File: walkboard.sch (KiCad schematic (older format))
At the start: 154 parts, among them J1 USB_C_Receptacle_USB2.0, SW1 SW_Push, U1 ATmega32U4-AU, Y1 Crystal_GND24_Small

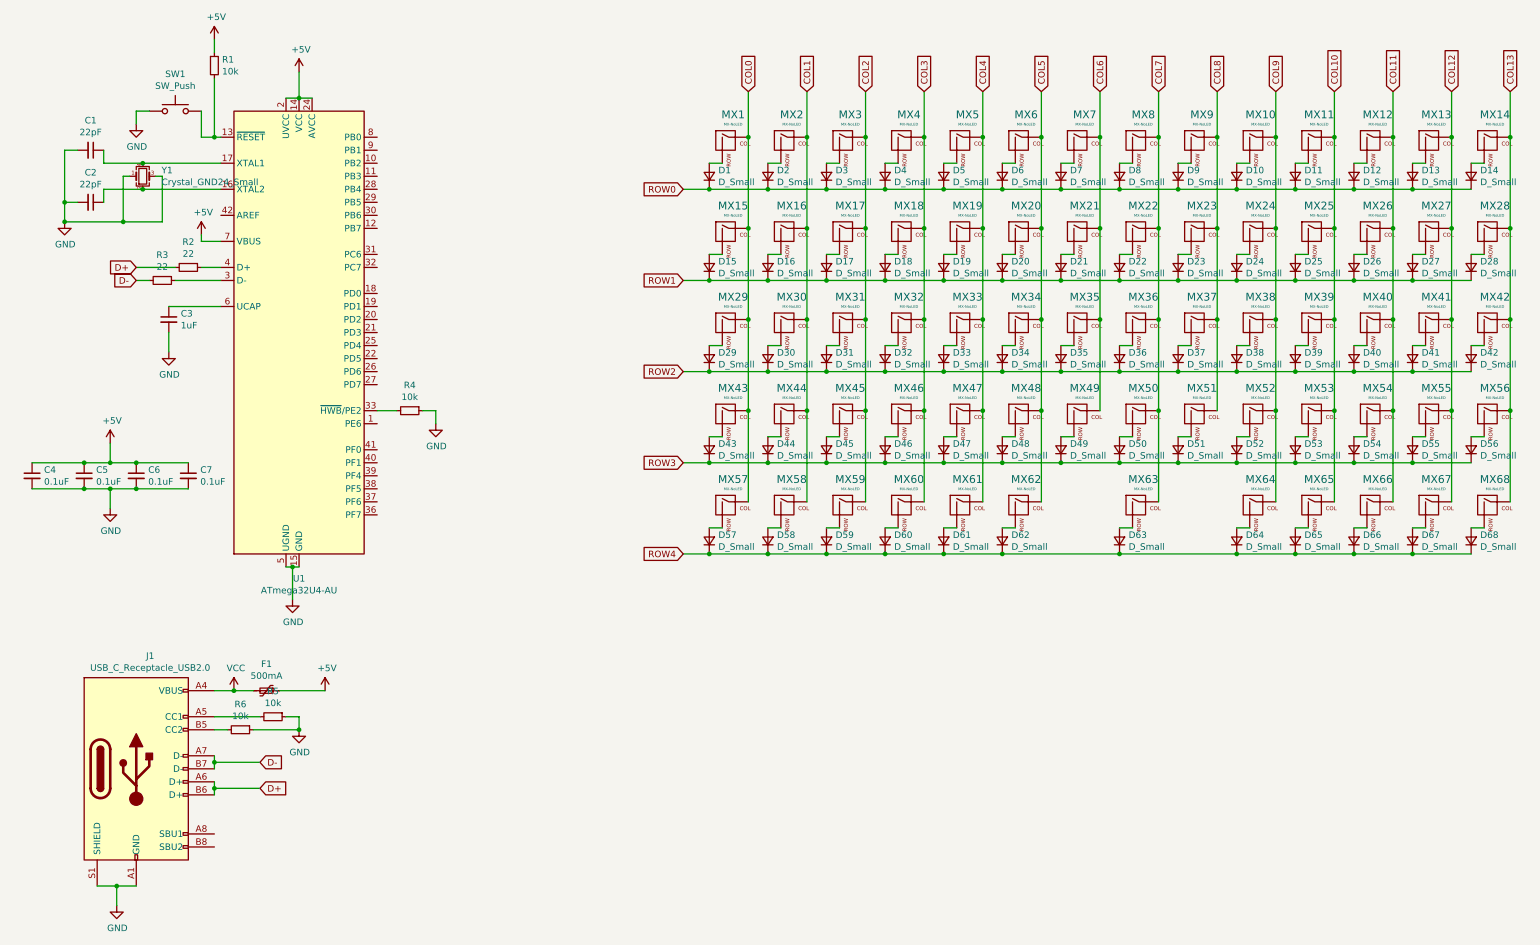
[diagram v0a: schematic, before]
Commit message: fixed
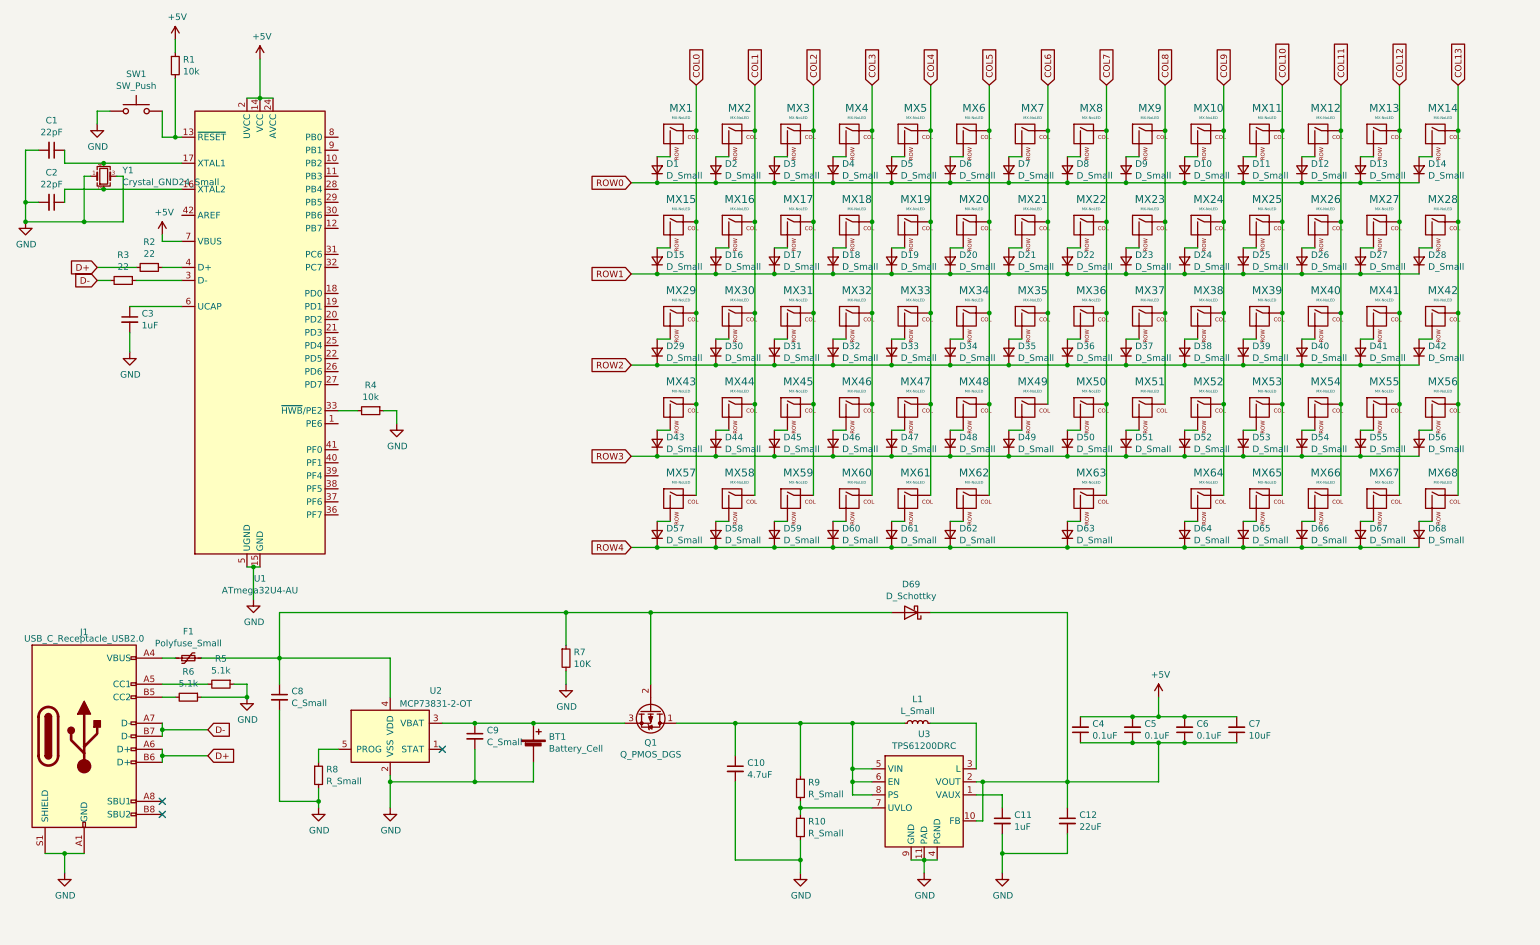
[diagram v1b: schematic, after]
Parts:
- added BT1: Battery_Cell, Connector_JST:JST_XH_S2B-XH-A_1x02_P2.50mm_Horizontal, symbol Device:Battery_Cell
- added C10: 4.7uF, Capacitor_SMD:C_0805_2012Metric_Pad1.15x1.40mm_HandSolder, symbol Device:C_Small
- added C11: 1uF, Capacitor_SMD:C_0805_2012Metric_Pad1.15x1.40mm_HandSolder, symbol Device:C_Small
- added C12: 22uF, Capacitor_SMD:C_0805_2012Metric_Pad1.15x1.40mm_HandSolder, symbol Device:C_Small
- added C8, C9: C_Small, Capacitor_SMD:C_0805_2012Metric_Pad1.15x1.40mm_HandSolder, symbol Device:C_Small
- added D69: D_Schottky, Diode_SMD:D_SOD-123, symbol Device:D_Schottky
- added L1: L_Small, Inductor_SMD:L_0805_2012Metric_Pad1.15x1.40mm_HandSolder, symbol Device:L_Small
- added Q1: Q_PMOS_DGS, Package_TO_SOT_SMD:SOT-23, symbol Device:Q_PMOS_DGS
- added R10, R8, R9: R_Small, Resistor_SMD:R_0805_2012Metric_Pad1.15x1.40mm_HandSolder, symbol Device:R_Small
- added R7: 10K, Resistor_SMD:R_0805_2012Metric_Pad1.15x1.40mm_HandSolder, symbol Device:R_Small
- added U2: MCP73831-2-OT, Package_TO_SOT_SMD:SOT-23-5, symbol Battery_Management:MCP73831-2-OT
- added U3: TPS61200DRC, Package_SON:Texas_S-PVSON-N10_ThermalVias, symbol Regulator_Switching:TPS61200DRC
- C7: value 0.1uF -> 10uF; footprint Diode_SMD:D_SOD-123 -> Capacitor_SMD:C_0805_2012Metric_Pad1.15x1.40mm_HandSolder
- F1: value 500mA -> Polyfuse_Small; footprint keyswitches:Kailh_socket_MX -> Fuse:Fuse_1206_3216Metric_Pad1.42x1.75mm_HandSolder
- MX68: footprint Resistor_SMD:R_0805_2012Metric -> keyswitches:Kailh_socket_MX
- R1, R2, R3, R4: footprint Resistor_SMD:R_0612_1632Metric_Pad1.18x3.40mm_HandSolder -> Resistor_SMD:R_0805_2012Metric_Pad1.15x1.40mm_HandSolder
- R5, R6: value 10k -> 5.1k; footprint Resistor_SMD:R_0612_1632Metric_Pad1.18x3.40mm_HandSolder -> Resistor_SMD:R_0805_2012Metric_Pad1.15x1.40mm_HandSolder
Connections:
- net +5V: now also C4.2, C5.2, C6.2, C7.2; no longer C4.1, C5.1, C6.1, C7.1, F1.1
- net GND: now also BT1.2 (-), C10.2, C11.2, C12.2, C8.2, C9.2, R10.2, R7.2, R8.2, U2.2 (VSS), U3.11 (PAD), U3.4 (PGND), U3.9 (GND); no longer C4.2, C5.2, C6.2, C7.2
- net VCC: no longer names the net of J1.A4 (VBUS), J1.A9 (VBUS), J1.B4 (VBUS), J1.B9 (VBUS)
- net VCC: now also F1.1; no longer F1.2
- new net: C11.1, U3.1 (VAUX)
- new net: C12.1, C4.1, C5.1, C6.1, C7.1, D69.1 (K), U3.10 (FB), U3.2 (VOUT)
- new net: L1.2, U3.3 (L)
- new net: C10.1, L1.1, Q1.1 (D), R9.1, U3.5 (VIN), U3.6 (EN), U3.8 (PS)
- new net: R10.1, R9.2, U3.7 (UVLO)
- new net: BT1.1 (+), C9.1, Q1.3 (S), U2.3 (VBAT)
- new net: C8.1, D69.2 (A), F1.2, Q1.2 (G), R7.1, U2.4 (VDD)
- new net: R8.1, U2.5 (PROG)
- no-connect marks 0 -> 3
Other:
- moved on the sheet: C1, C2, C3, D1, D10, D11, D12, D13, D14, D15, D16, D17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
